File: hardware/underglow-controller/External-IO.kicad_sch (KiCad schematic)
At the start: 70 parts, among them Q601 STS8DNF3LL, Q602 STS8DNF3LL, Q603 STS8DNF3LL, Q604 SBC847CDW1T1G, Q605 SBC847CDW1T1G, Q606 AUIRF7316QTR, Q607 STS8DNF3LL, U601 INA2181A1IDGST, U602 ZXGD3009E6, U603 ZXGD3009E6, U604 ZXGD3009E6, U605 ZXGD3009E6, U606 ZXGD3009E6, U607 ZXGD3009E6, U608 ZXGD3009E6, U609 ZXGD3009E6

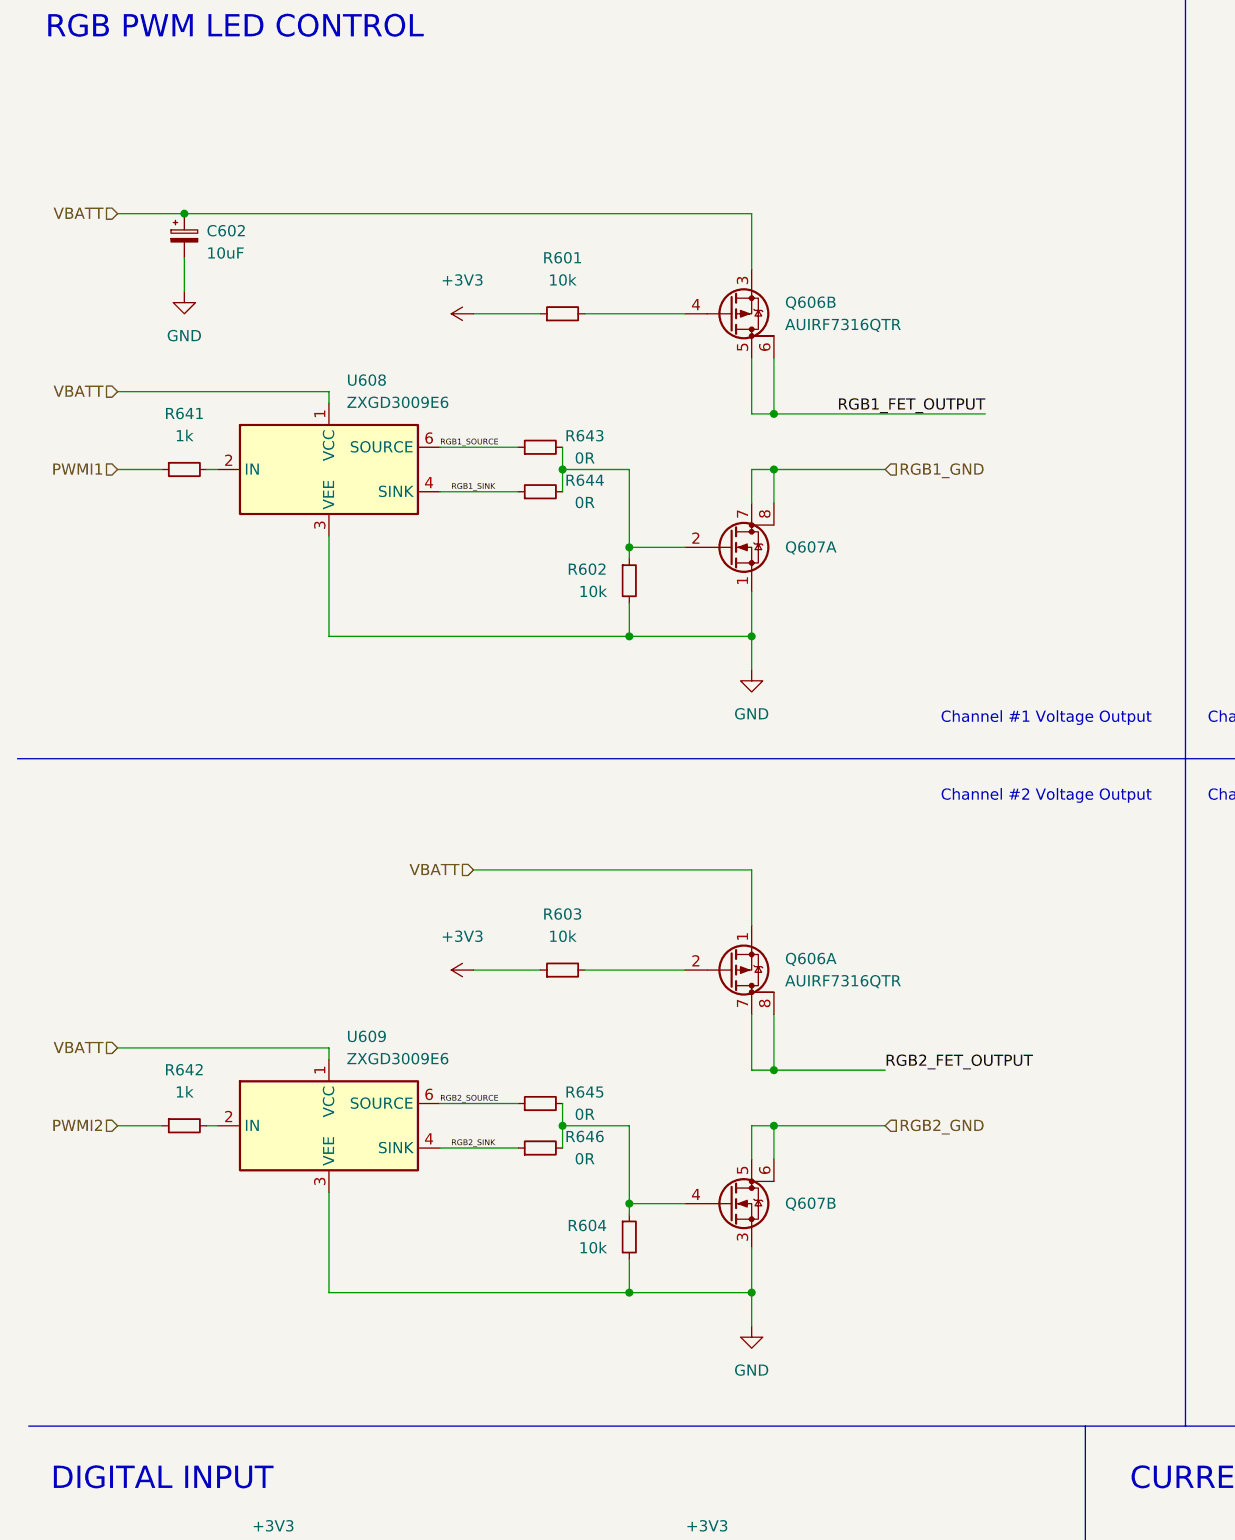
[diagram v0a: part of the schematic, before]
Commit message: hw updates based on latest boards
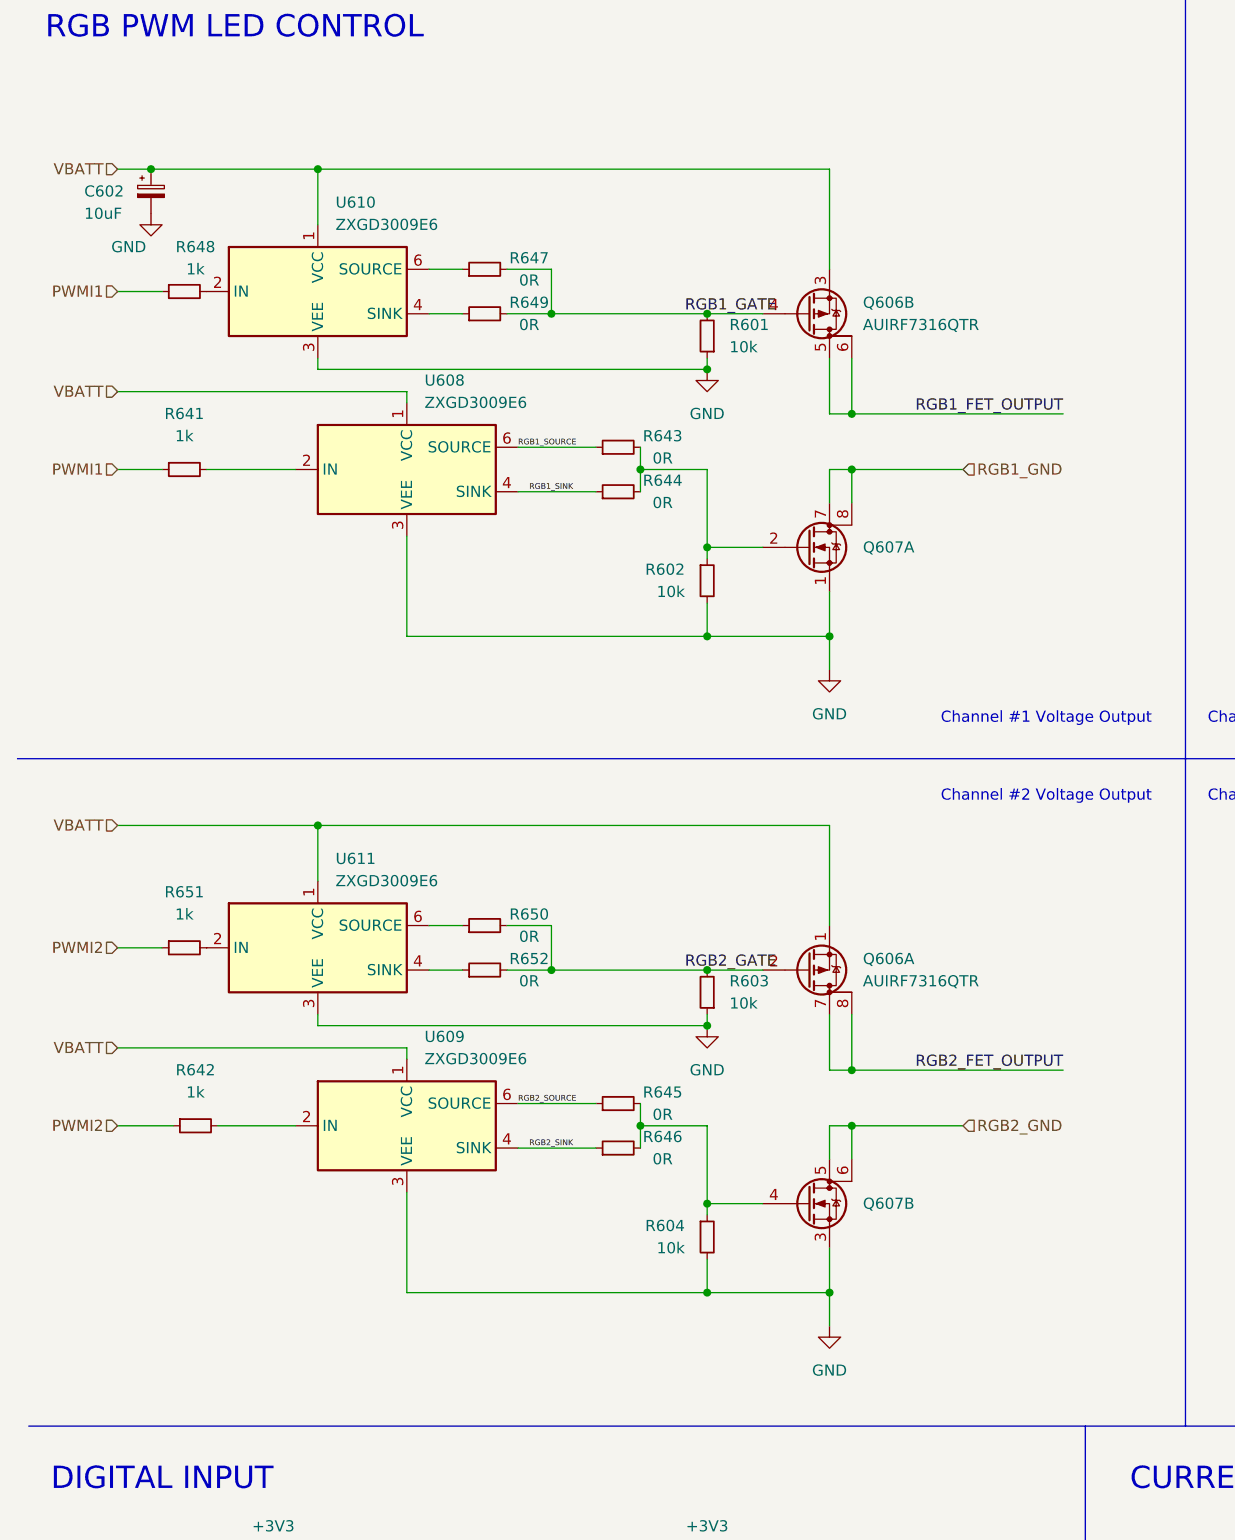
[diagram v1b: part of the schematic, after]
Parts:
- added R647, R649, R650, R652: 0R, Resistor_SMD:R_0805_2012Metric, symbol Device:R_Small
- added R648, R651: 1k, Resistor_SMD:R_0402_1005Metric, symbol Device:R_Small
- added U610, U611: ZXGD3009E6, Package_TO_SOT_SMD:SOT-23-6, symbol Driver_FET:ZXGD3009E6
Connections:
- net +3V3: no longer R601.1, R603.1
- net GND: now also R601.1, R603.1, U610.3 (VEE), U611.3 (VEE)
- net PWMI1: now also R648.1
- net PWMI2: now also R651.1
- net VBATT: now also U610.1 (VCC), U611.1 (VCC)
- net RGB1_GATE: now reaches Q606.4 (G), R601.2
- net RGB1_GATE: now also R647.2, R649.2
- net RGB2_GATE: now reaches Q606.2 (G), R603.2
- net RGB2_GATE: now also R650.2, R652.2
- new net: R649.1, U610.4 (SINK)
- new net: R650.1, U611.6 (SOURCE)
- new net: R648.2, U610.2 (IN)
- new net: R647.1, U610.6 (SOURCE)
- new net: R651.2, U611.2 (IN)
- new net: R652.1, U611.4 (SINK)
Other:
- moved on the sheet: C602, Q606A, Q606B, Q607A, Q607B, R601, R602, R603, R604, R642, R643, R644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

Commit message: https://www.youtube.com/watch?v=FZUcpVmEHuk&ab_channel=billwurtz
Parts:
- R629, R630, R631, R632, R633, R634, R635, R636, R637, R638, R639, R640, R643, R644, R645, R646, R647, R649, R650, R652: MPN (none) -> RES SMD 0 OHM JUMPER 1/8W 0805
- U602, U603, U604, U605, U606, U607, U608, U609, U610, U611: MPN (none) -> ZXGD3009E6
